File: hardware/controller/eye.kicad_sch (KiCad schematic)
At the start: 25 parts, among them U4 EMS4000RSW, U5 baochip1x, Y1 48 MHz

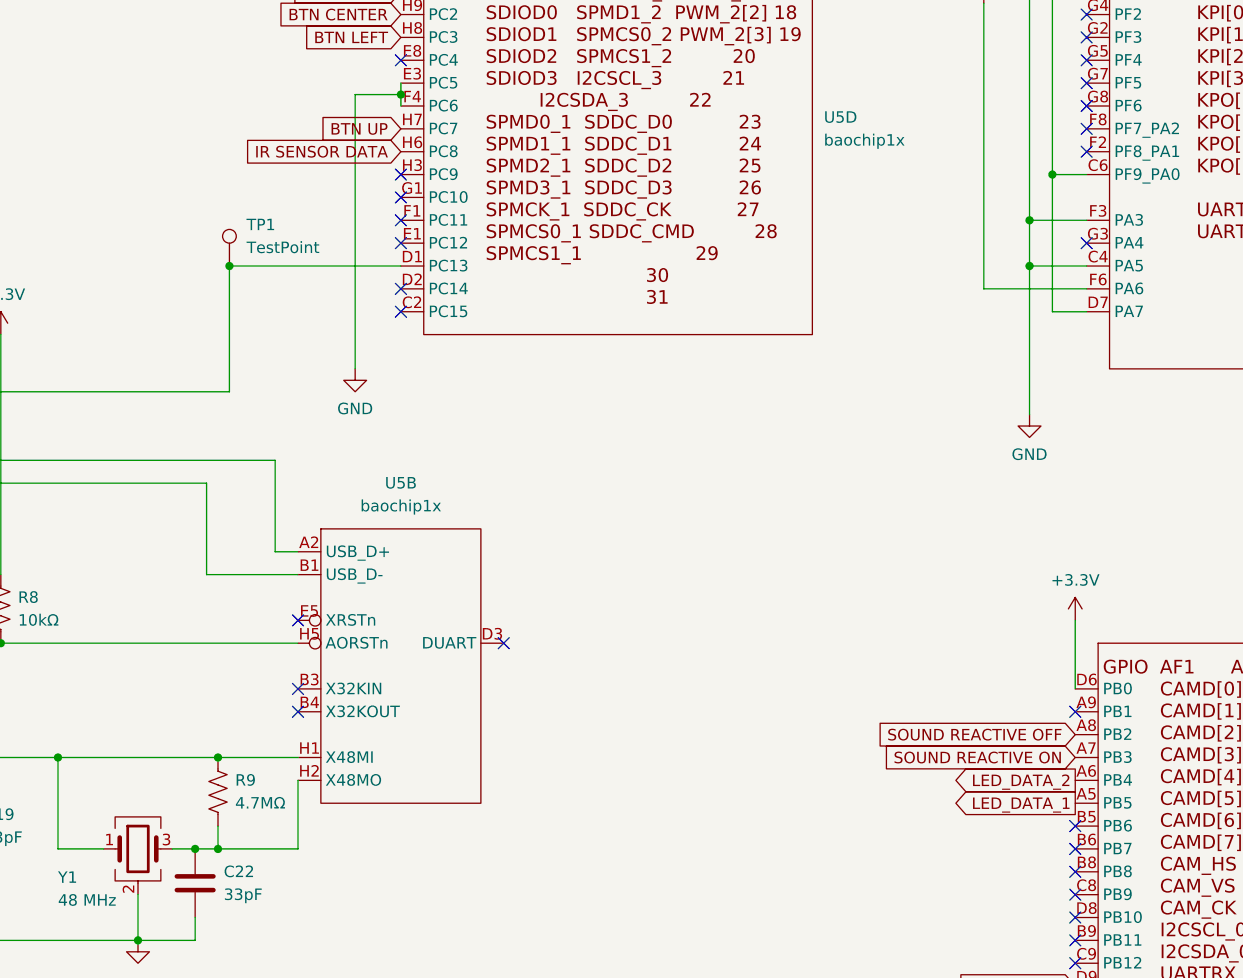
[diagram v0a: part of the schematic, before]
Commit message: routing adjustments/fixes
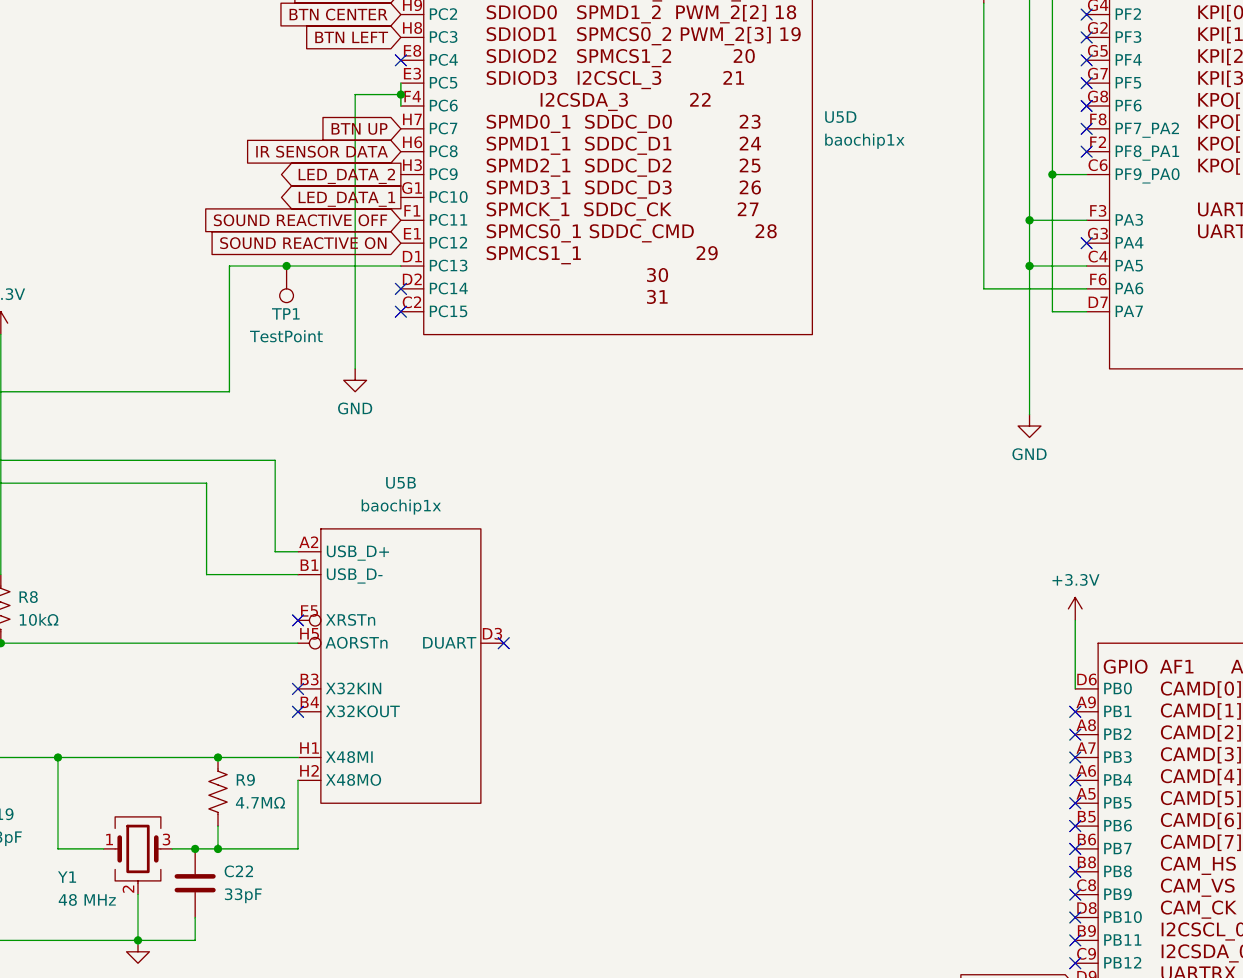
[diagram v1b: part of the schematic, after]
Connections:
- net LED_DATA_1: now also U5.G1 (PC10); no longer U5.A5 (PB5)
- net LED_DATA_2: now also U5.H3 (PC9); no longer U5.A6 (PB4)
- net SOUND REACTIVE OFF: now also U5.F1 (PC11); no longer U5.A8 (PB2)
- net SOUND REACTIVE ON: now also U5.E1 (PC12); no longer U5.A7 (PB3)
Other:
- moved on the sheet: TP1
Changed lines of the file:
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@@
 	)
 	(junction
-		(at 128.27 62.23)
+		(at 134.62 62.23)
 		(diameter 0)
 		(color 0 0 0 0)
@@
 	)
 	(no_connect
-		(at 147.32 59.69)
+		(at 222.25 116.84)
 	)
 	(no_connect
@@
 	)
 	(no_connect
-		(at 147.32 54.61)
+		(at 222.25 121.92)
 	)
 	(no_connect
@@
 	)
 	(no_connect
-		(at 147.32 57.15)
+		(at 222.25 114.3)
 	)
 	(no_connect
@@
 	)
 	(no_connect
-		(at 147.32 52.07)
+		(at 222.25 119.38)
 	)
 	(no_connect
@@
 	(wire
 		(pts
-			(xy 128.27 62.23) (xy 147.32 62.23)
+			(xy 128.27 62.23) (xy 134.62 62.23)
+		)
+		(stroke
+			(width 0)
+			(type default)
+		)
+	)
+	(wire
+		(pts
+			(xy 134.62 62.23) (xy 147.32 62.23)
 		)
 		(stroke
@@
 	(global_label "LED_DATA_2"
 		(shape output)
-		(at 222.25 119.38 180)
+		(at 147.32 52.07 180)
 		(fields_autoplaced yes)
 		(effects
@@
 		)
 		(property "Intersheetrefs" "${INTERSHEET_REFS}"
-			(at 208.2582 119.38 0)
+			(at 133.33 52.07 0)
 			(hide yes)
 			(show_name no)
@@
 	(global_label "SOUND REACTIVE ON"
 		(shape input)
-		(at 222.25 116.84 180)
+		(at 147.32 59.69 180)
 		(fields_autoplaced yes)
 		(effects
@@
 		)
 		(property "Intersheetrefs" "${INTERSHEET_REFS}"
-			(at 199.61 116.84 0)
+			(at 124.68 59.69 0)
 			(hide yes)
 			(show_name no)
@@
 	(global_label "LED_DATA_1"
 		(shape output)
-		(at 222.25 121.92 180)
+		(at 147.32 54.61 180)
 		(fields_autoplaced yes)
 		(effects
@@
 		)
 		(property "Intersheetrefs" "${INTERSHEET_REFS}"
-			(at 208.2582 121.92 0)
+			(at 133.33 54.61 0)
 			(hide yes)
 			(show_name no)
@@
 	(global_label "SOUND REACTIVE OFF"
 		(shape input)
-		(at 222.25 114.3 180)
+		(at 147.32 57.15 180)
 		(fields_autoplaced yes)
 		(effects
@@
 		)
 		(property "Intersheetrefs" "${INTERSHEET_REFS}"
-			(at 198.7633 114.3 0)
+			(at 123.83 57.15 0)
 			(hide yes)
 			(show_name no)
@@
 	(symbol
 		(lib_id "Connector:TestPoint")
-		(at 128.27 62.23 0)
+		(at 134.62 62.23 180)
 		(unit 1)
 		(body_style 1)
@@
 		(fields_autoplaced yes)
 		(property "Reference" "TP1"
-			(at 130.175 57.6579 0)
+			(at 134.62 67.6 0)
 			(show_name no)
 			(do_not_autoplace no)
@@
 					(size 1.27 1.27)
 				)
-				(justify left)
 			)
 		)
 		(property "Value" "TestPoint"
-			(at 130.175 60.1979 0)
+			(at 134.62 70.1 0)
 			(show_name no)
 			(do_not_autoplace no)
@@
 					(size 1.27 1.27)
 				)
-				(justify left)
 			)
 		)
 		(property "Footprint" "TestPoint:TestPoint_Pad_D1.0mm"
-			(at 133.35 62.23 0)
+			(at 139.7 62.23 0)
 			(hide yes)
 			(show_name no)
@@
 		)
 		(property "Datasheet" ""
-			(at 133.35 62.23 0)
+			(at 139.7 62.23 0)
 			(hide yes)
 			(show_name no)
@@
 		)
 		(property "Description" "test point"
-			(at 128.27 62.23 0)
+			(at 134.62 62.23 0)
 			(hide yes)
 			(show_name no)
